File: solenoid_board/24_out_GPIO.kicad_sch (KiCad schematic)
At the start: 120 parts, among them J1 mx2.54, J10 mx2.54, J13 mx2.54, J14 mx2.54, J17 mx2.54, J18 mx2.54, J2 mx2.54, J5 mx2.54, J6 mx2.54, J9 mx2.54, Q1 IRF540NSTRLPBF, Q10 IRF540NSTRLPBF, Q2 IRF540NSTRLPBF, Q3 IRF540NSTRLPBF, Q4 IRF540NSTRLPBF, Q5 IRF540NSTRLPBF, Q6 IRF540NSTRLPBF, Q7 IRF540NSTRLPBF, Q8 IRF540NSTRLPBF, Q9 IRF540NSTRLPBF, SW1 SW_Push, SW10 SW_Push, SW2 SW_Push, SW3 SW_Push, SW4 SW_Push, SW5 SW_Push, SW6 SW_Push, SW7 SW_Push, SW8 SW_Push, SW9 SW_Push, U10 4N35, U11 4N35, U12 4N35, U3 4N35, U4 4N35, U5 4N35, U6 4N35, U7 4N35, U8 4N35, U9 4N35

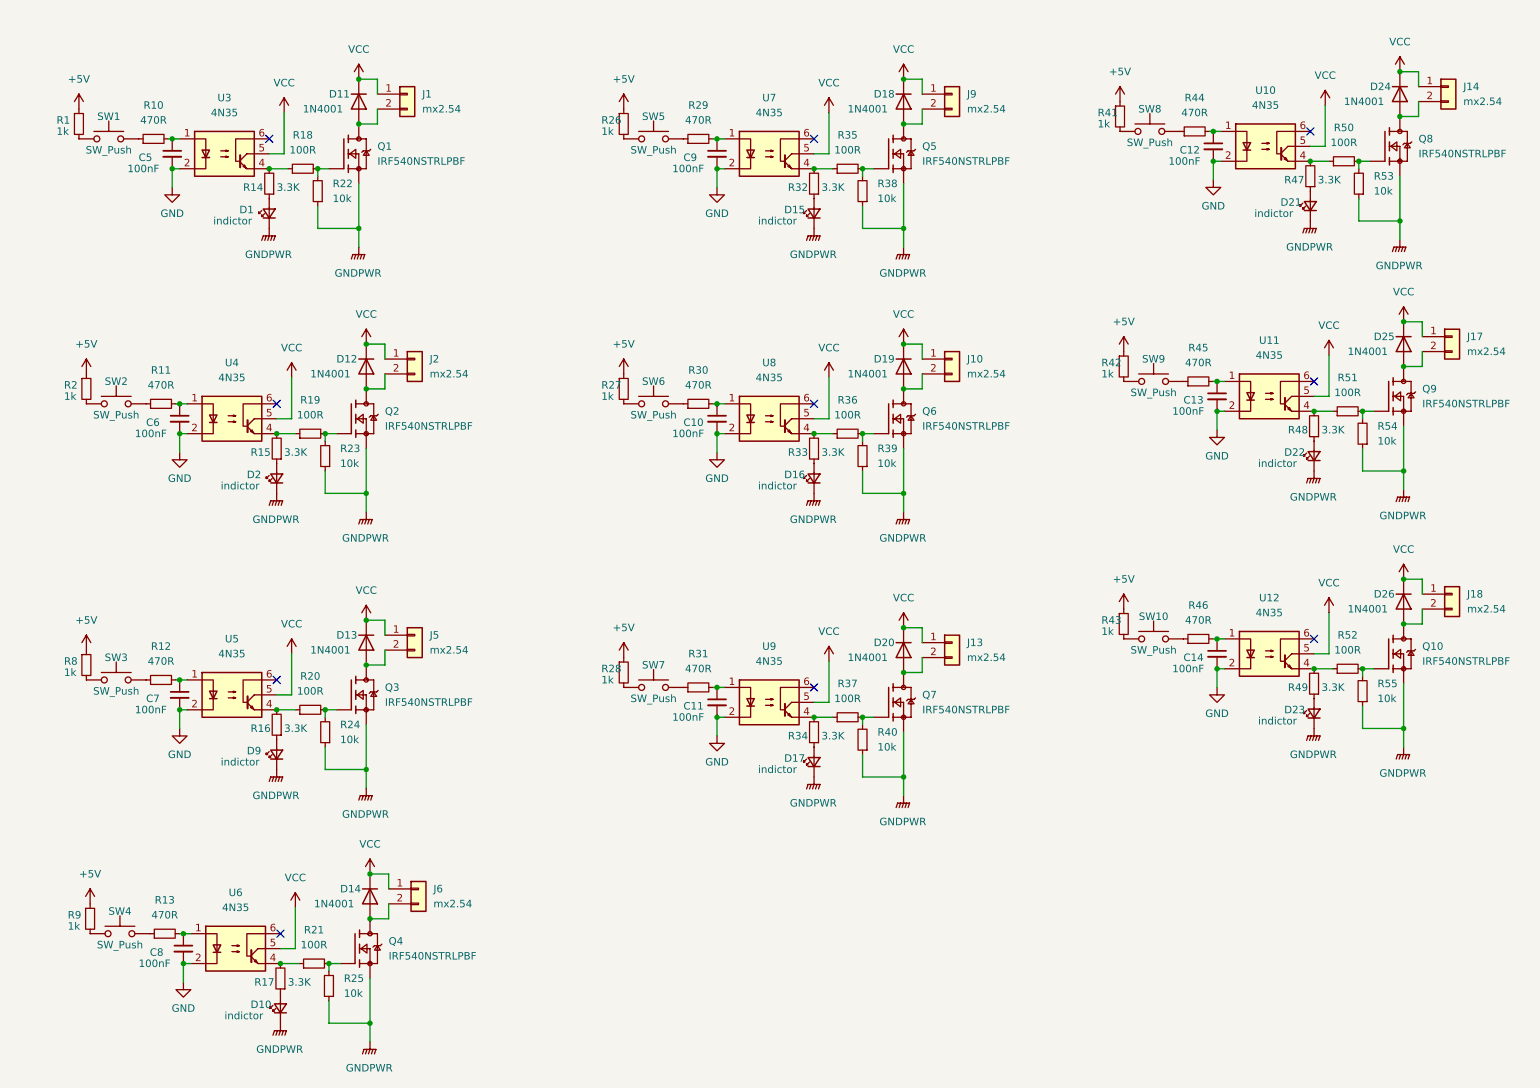
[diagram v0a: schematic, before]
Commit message: add
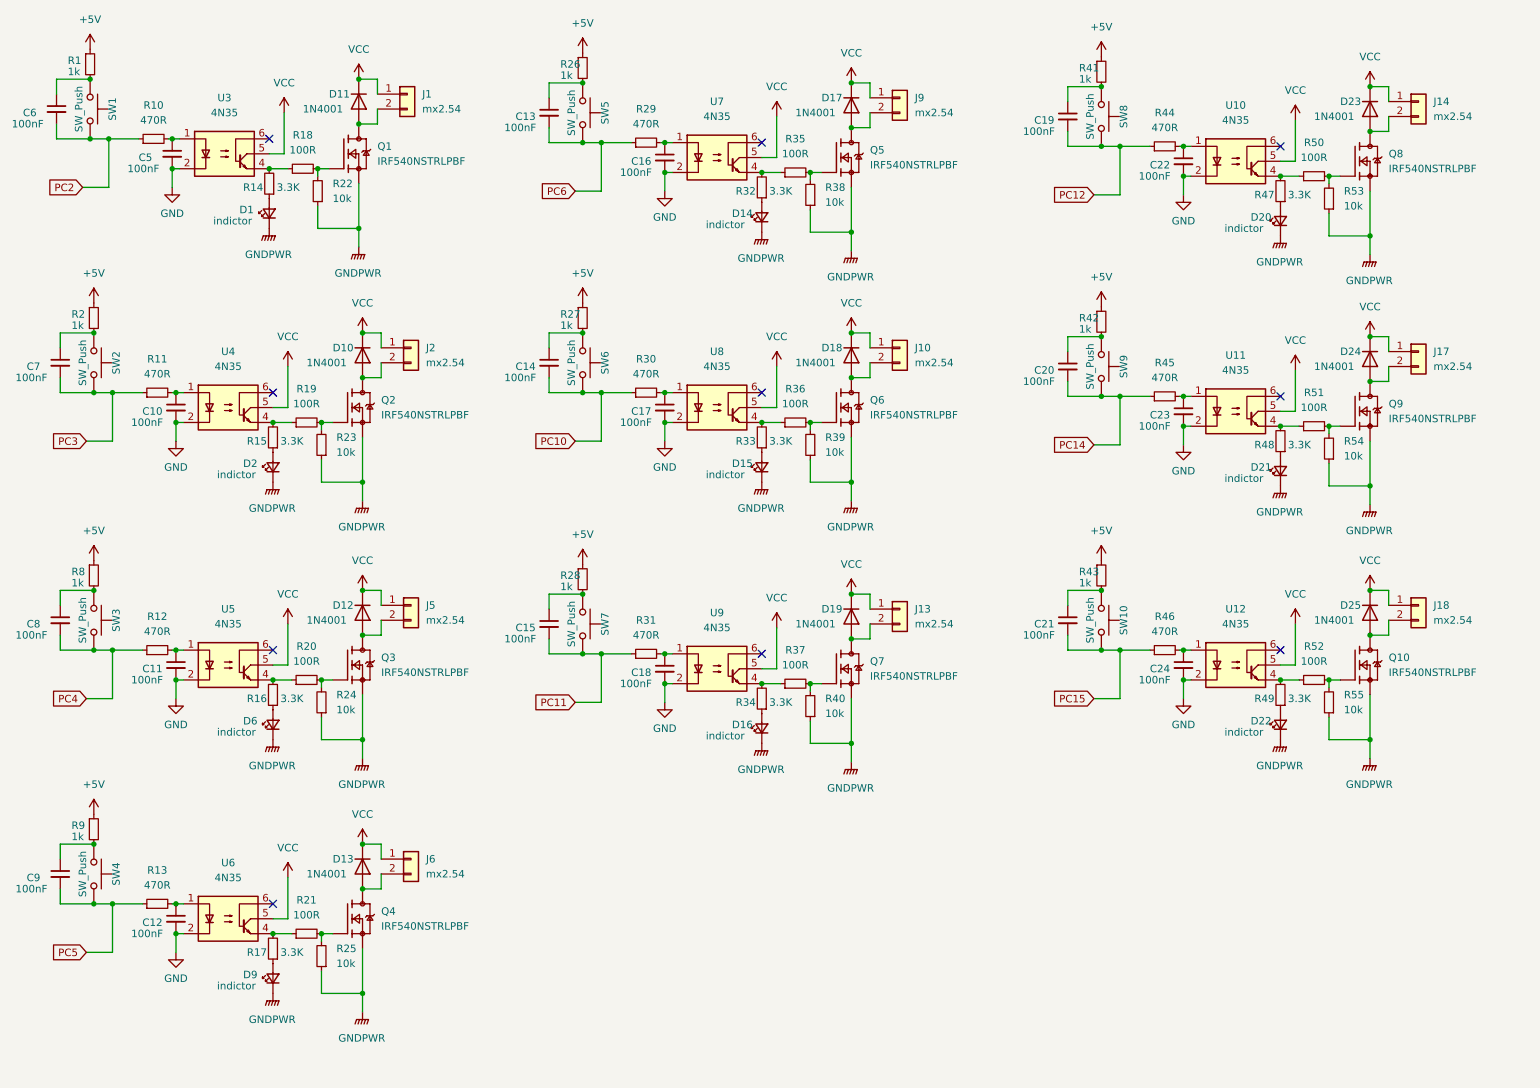
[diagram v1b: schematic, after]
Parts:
- removed D10, D17, D23: indictor, symbol Device:LED_Small
- removed D14, D20, D26: 1N4001, Diode_THT:D_DO-41_SOD81_P10.16mm_Horizontal, symbol Diode:1N4001
- added C15, C16, C17, C18, C19, C20, C21, C22, C23, C24: 100nF, Capacitor_SMD:C_0805_2012Metric_Pad1.18x1.45mm_HandSolder, symbol Device:C_Small
- added D10, D17, D23: 1N4001, Diode_THT:D_DO-41_SOD81_P10.16mm_Horizontal, symbol Diode:1N4001
- added D14, D20, D6: indictor, LED_SMD:LED_0805_2012Metric_Pad1.15x1.40mm_HandSolder, symbol Device:LED_Small
- C10, C11, C12, C13, C14, C5, C6, C7, C8, C9: footprint (none) -> Capacitor_SMD:C_0805_2012Metric_Pad1.18x1.45mm_HandSolder
- D1, D15, D16, D2, D21, D22, D9: footprint (none) -> LED_SMD:LED_0805_2012Metric_Pad1.15x1.40mm_HandSolder
- J1, J10, J13, J14, J17, J18, J2, J5, J6, J9: footprint (none) -> Connector_PinHeader_2.54mm:PinHeader_1x02_P2.54mm_Vertical
- R1, R10, R11, R12, R13, R14, R15, R16, R17, R18, R19, R2, R20, R21, R22, R23, R24, R25, R26, R27, R28, R29, R30, R31, R32, R33, R34, R35, R36, R37, R38, R39, R40, R41, R42, R43, R44, R45, R46, R47, R48, R49, R50, R51, R52, R53, R54, R55, R8, R9: footprint (none) -> Resistor_SMD:R_0805_2012Metric_Pad1.20x1.40mm_HandSolder
- SW1, SW10, SW2, SW3, SW4, SW5, SW6, SW7, SW8, SW9: footprint (none) -> Button_Switch_SMD:SW_SPST_TL3305A
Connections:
- net GND: now also C16.2, C17.2, C18.2, C22.2, C23.2, C24.2; no longer C13.2, C14.2, C6.2, C7.2, C8.2, C9.2
- net GNDPWR: now also D14.1 (K), D20.1 (K), D6.1 (K)
- net VCC: now also D10.1 (K), D17.1 (K), D23.1 (K)
- net at J6.2 (Pin_2), Q4.2: now also D13.2 (A)
- net at J10.2 (Pin_2), Q6.2: now also D18.2 (A); no longer D19.2 (A)
- net PC6: now reaches R29.1, SW5.2
- net PC6: now also C13.2
- net at R29.2, U7.1: now also C16.1; no longer C9.1
- net at R42.2, SW9.1: now also C20.1
- net at R43.2, SW10.1: now also C21.1
- net PC15: now reaches R46.1, SW10.2
- net PC15: now also C21.2
- net at R28.2, SW7.1: now also C15.1
- net at R31.2, U9.1: now also C18.1; no longer C11.1
- net at J9.2 (Pin_2), Q5.2: now also D17.2 (A); no longer D18.2 (A)
- net at R30.2, U8.1: now also C17.1; no longer C10.1
- net at R49.1: now also D22.2 (A)
- net PC3: now reaches R11.1, SW2.2
- net PC3: now also C7.2
- net at R11.2, U4.1: now also C10.1; no longer C6.1
- net at R48.1: now also D21.2 (A); no longer D22.2 (A)
- net at J2.2 (Pin_2), Q2.2: now also D10.2 (A); no longer D12.2 (A)
- net at R47.1: now also D20.2 (A); no longer D21.2 (A)
- net at D9.2 (A): now also R17.1; no longer R16.1
- net at J13.2 (Pin_2), Q7.2: now also D19.2 (A)
- net at R45.2, U11.1: now also C23.1; no longer C13.1
- net PC5: now reaches R13.1, SW4.2
- net PC5: now also C9.2
- net at R13.2, U6.1: now also C12.1; no longer C8.1
- net at R26.2, SW5.1: now also C13.1
- net at J18.2 (Pin_2), Q10.2: now also D25.2 (A)
- net at R34.1: now also D16.2 (A)
- net at R8.2, SW3.1: now also C8.1
- net at R46.2, U12.1: now also C24.1; no longer C14.1
- net at R33.1: now also D15.2 (A); no longer D16.2 (A)
- net at R1.2, SW1.1: now also C6.1
- net at R2.2, SW2.1: now also C7.1
- net at R32.1: now also D14.2 (A); no longer D15.2 (A)
- net at J14.2 (Pin_2), Q8.2: now also D23.2 (A); no longer D24.2 (A)
- net at R44.2, U10.1: now also C22.1; no longer C12.1
- net at J5.2 (Pin_2), Q3.2: now also D12.2 (A); no longer D13.2 (A)
- net PC2: now reaches R10.1, SW1.2
- net PC2: now also C6.2
- net at R12.2, U5.1: now also C11.1; no longer C7.1
- net PC4: now reaches R12.1, SW3.2
- net PC4: now also C8.2
- net at J17.2 (Pin_2), Q9.2: now also D24.2 (A); no longer D25.2 (A)
- net at R27.2, SW6.1: now also C14.1
- net PC11: now reaches R31.1, SW7.2
- net PC11: now also C15.2
- net at R41.2, SW8.1: now also C19.1
- net PC12: now reaches R44.1, SW8.2
- net PC12: now also C19.2
- net at R9.2, SW4.1: now also C9.1
- net PC10: now reaches R30.1, SW6.2
- net PC10: now also C14.2
- net PC14: now reaches R45.1, SW9.2
- net PC14: now also C20.2
- new net: D6.2 (A), R16.1
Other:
- moved on the sheet: R1, SW1
